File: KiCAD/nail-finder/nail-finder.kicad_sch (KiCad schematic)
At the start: 29 parts, among them J12 ST-LINK, J13 batt.-F, J14 batt.-M, J15 speaker-F, J16 speaker-M, Q2 ZTX649, SW5 reset, SW6 power, U2 STM8S103F3M, Y3 12Mhz

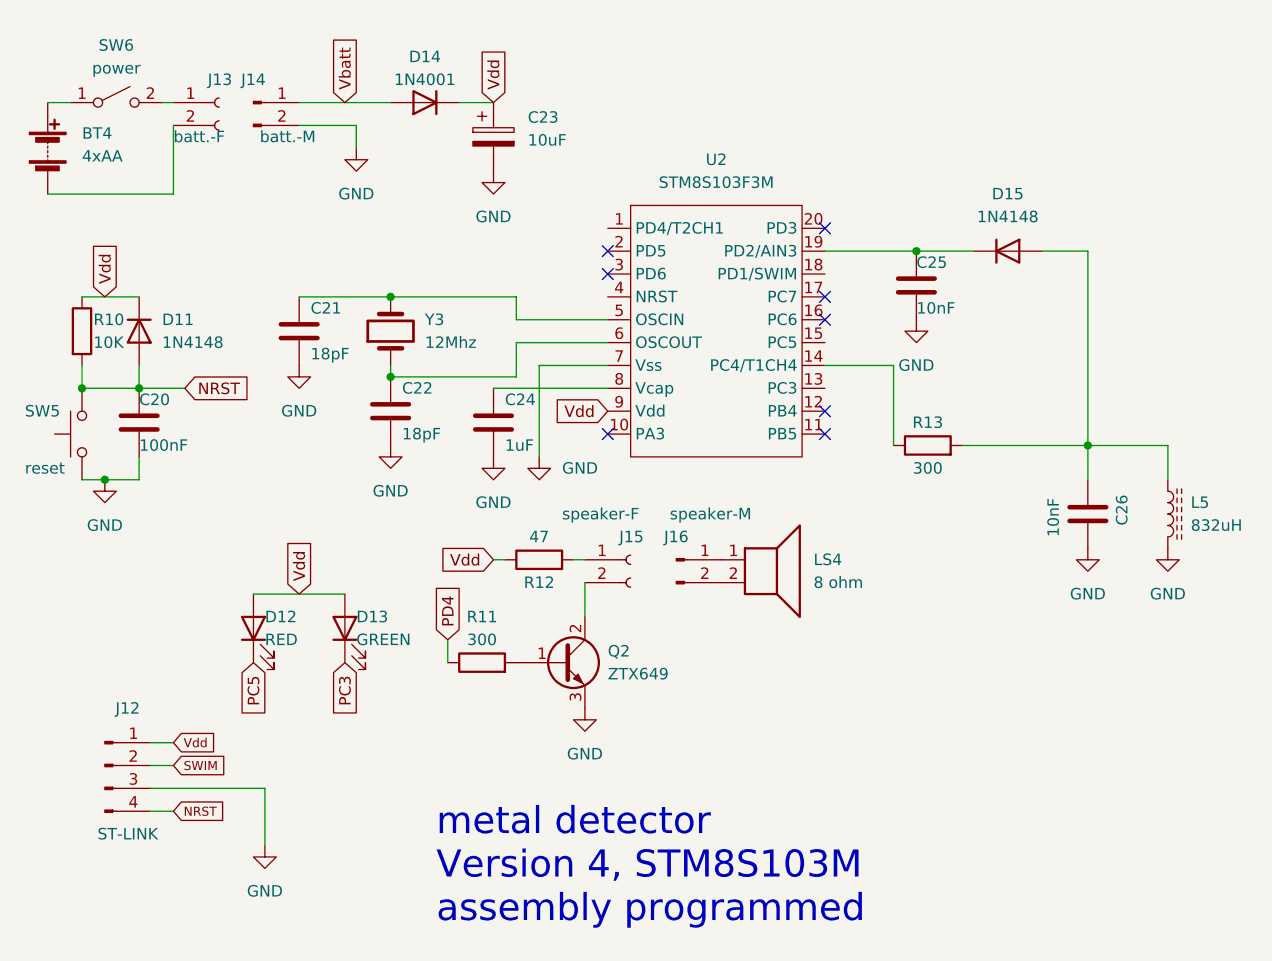
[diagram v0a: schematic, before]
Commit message: circuit final choisi nail-finder.v7.png
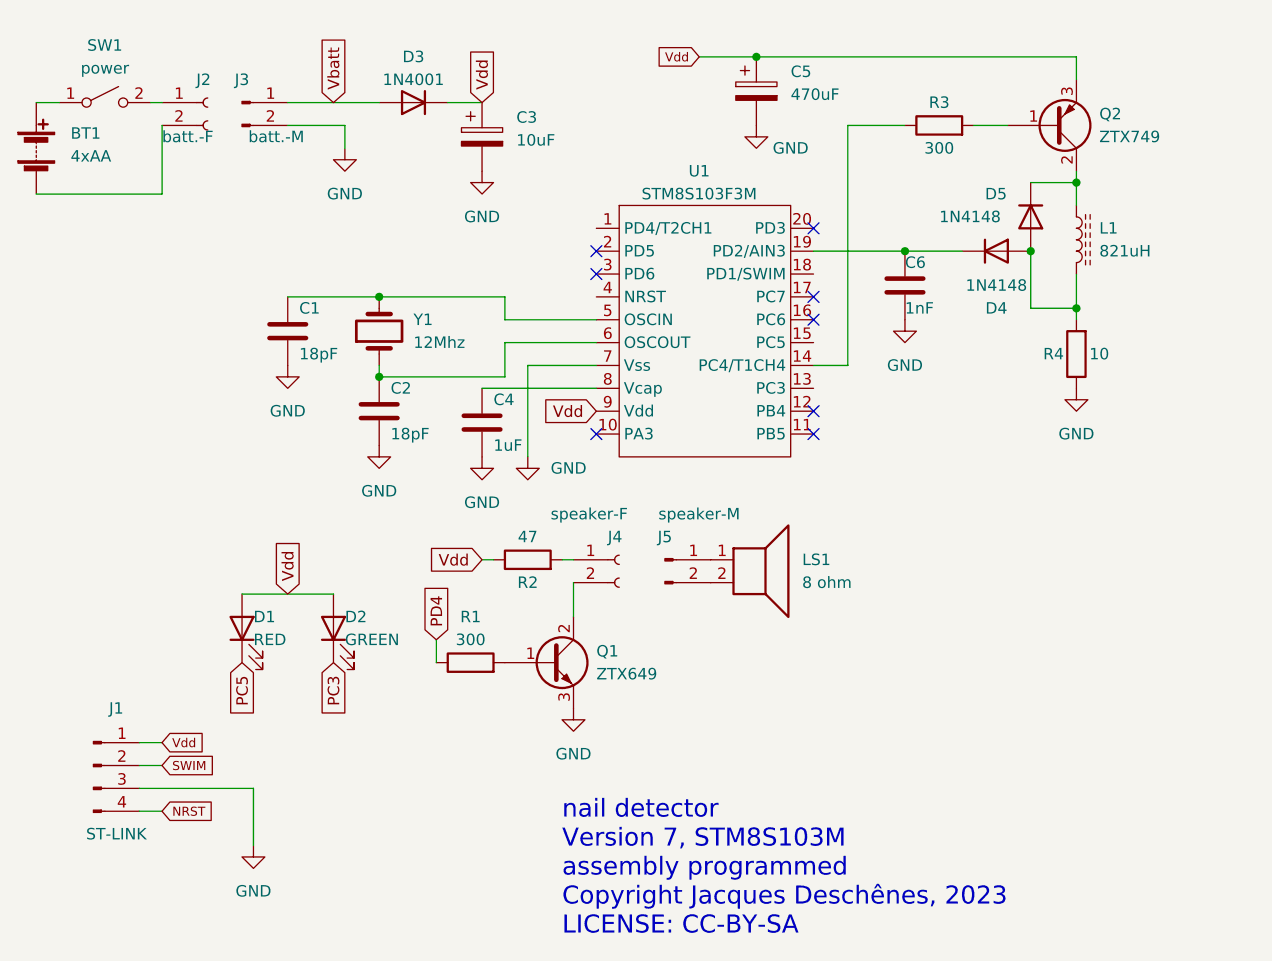
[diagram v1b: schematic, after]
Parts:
- removed BT4: 4xAA, symbol Device:Battery
- removed C20: 100nF, symbol Device:C
- removed C21, C22: 18pF, symbol Device:C
- removed C23: 10uF, symbol Device:C_Polarized
- removed C24: 1uF, symbol Device:C
- removed C25, C26: 10nF, symbol Device:C
- removed D11, D15: 1N4148, Diode_THT:D_DO-35_SOD27_P7.62mm_Horizontal, symbol Diode:1N4148
- removed D12: RED, symbol Device:LED
- removed D13: GREEN, symbol Device:LED
- removed D14: 1N4001, Diode_THT:D_DO-41_SOD81_P10.16mm_Horizontal, symbol Diode:1N4001
- removed J12: ST-LINK, symbol Connector:Conn_01x04_Male
- removed J13: batt.-F, symbol Connector:Conn_01x02_Female
- removed J14: batt.-M, symbol Connector:Conn_01x02_Male
- removed J15: speaker-F, symbol Connector:Conn_01x02_Female
- removed J16: speaker-M, symbol Connector:Conn_01x02_Male
- removed L5: 832uH, symbol Device:L_Ferrite
- removed LS4: 8 ohm, symbol Device:Speaker
- removed Q2: ZTX649, symbol Device:Q_NPN_BCE
- removed R10: 10K, symbol Device:R
- removed R11, R13: 300, symbol Device:R
- removed R12: 47, symbol Device:R
- removed SW5: reset, symbol Switch:SW_MEC_5G
- removed SW6: power, symbol Switch:SW_SPST
- removed U2: STM8S103F3M, symbol MCU_ST_STM8:STM8S103F3M
- removed Y3: 12Mhz, symbol Device:Crystal
- added BT1: 4xAA, symbol Device:Battery
- added C1, C2: 18pF, symbol Device:C
- added C3: 10uF, symbol Device:C_Polarized
- added C4: 1uF, symbol Device:C
- added C5: 470uF, symbol Device:C_Polarized
- added C6: 1nF, symbol Device:C
- added D1: RED, symbol Device:LED
- added D2: GREEN, symbol Device:LED
- added D3: 1N4001, Diode_THT:D_DO-41_SOD81_P10.16mm_Horizontal, symbol Diode:1N4001
- added D4, D5: 1N4148, Diode_THT:D_DO-35_SOD27_P7.62mm_Horizontal, symbol Diode:1N4148
- added J1: ST-LINK, symbol Connector:Conn_01x04_Male
- added J2: batt.-F, symbol Connector:Conn_01x02_Female
- added J3: batt.-M, symbol Connector:Conn_01x02_Male
- added J4: speaker-F, symbol Connector:Conn_01x02_Female
- added J5: speaker-M, symbol Connector:Conn_01x02_Male
- added L1: 821uH, symbol Device:L_Ferrite
- added LS1: 8 ohm, symbol Device:Speaker
- added Q1: ZTX649, symbol Device:Q_NPN_BCE
- added Q2: ZTX749, symbol Device:Q_PNP_BCE
- added R1, R3: 300, symbol Device:R
- added R2: 47, symbol Device:R
- added R4: 10, symbol Device:R
- added SW1: power, symbol Switch:SW_SPST
- added U1: STM8S103F3M, symbol MCU_ST_STM8:STM8S103F3M
- added Y1: 12Mhz, symbol Device:Crystal
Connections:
- net GND: now also C1.2, C2.2, C3.2, C4.2, C5.2, C6.2, J1.3 (Pin_3), J3.2 (Pin_2), Q1.3 (E), R4.1, U1.7 (Vss)
- net NRST: now also J1.4 (Pin_4)
- net PC3: now also D2.1 (K)
- net PC5: now also D1.1 (K)
- net PD4: now also R1.1
- net SWIM: now also J1.2 (Pin_2)
- net Vbatt: now also D3.2 (A), J3.1 (Pin_1)
- net Vdd: now also C3.1, C5.1, D1.2 (A), D2.2 (A), D3.1 (K), J1.1 (Pin_1), Q2.3 (E), R2.1, U1.9 (Vdd)
- new net: J4.1 (Pin_1), R2.2
- new net: C4.1, U1.8 (Vcap)
- new net: Q1.1 (B), R1.2
- new net: J2.1 (Pin_1), SW1.2 (B)
- new net: BT1.2 (-), J2.2 (Pin_2)
- new net: C1.1, U1.5 (OSCIN), Y1.2
- new net: C2.1, U1.6 (OSCOUT), Y1.1
- new net: J4.2 (Pin_2), Q1.2 (C)
- new net: D4.2 (A), D5.2 (A), L1.2, R4.2
- new net: R3.1, U1.14 (PC4/T1CH4)
- new net: C6.1, D4.1 (K), U1.19 (PD2/AIN3)
- new net: BT1.1 (+), SW1.1 (A)
- new net: J5.1 (Pin_1), LS1.1
- new net: J5.2 (Pin_2), LS1.2
- new net: Q2.1 (B), R3.2
- new net: D5.1 (K), L1.1, Q2.2 (C)
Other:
- note added: "nail detector Version 7, STM8S103M assembly programmed Copyright Jacques Deschênes, 2023 LICENSE: CC-BY-SA"
- note removed: "metal detector Version 4, STM8S103M assembly programmed"
